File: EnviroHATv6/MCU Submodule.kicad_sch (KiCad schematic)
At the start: 10 parts, among them J1 Conn_01x10_Pin, J2 Conn_01x32_Socket, J3 Conn_01x32_Socket, U1 STM32F051R8Tx, U2 FT234XD-R, U3 CAT24C256

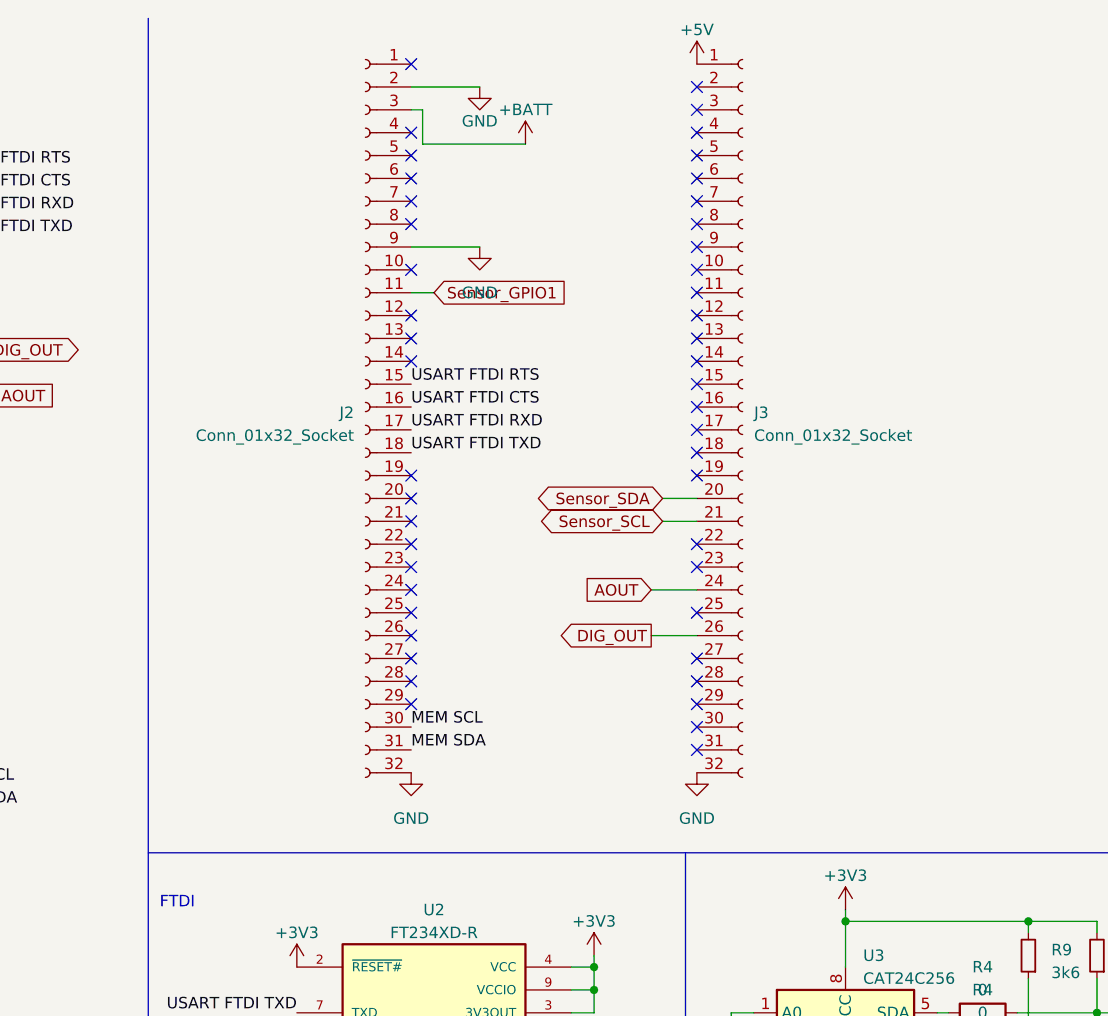
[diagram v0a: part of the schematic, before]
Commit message: Update to v 6.2
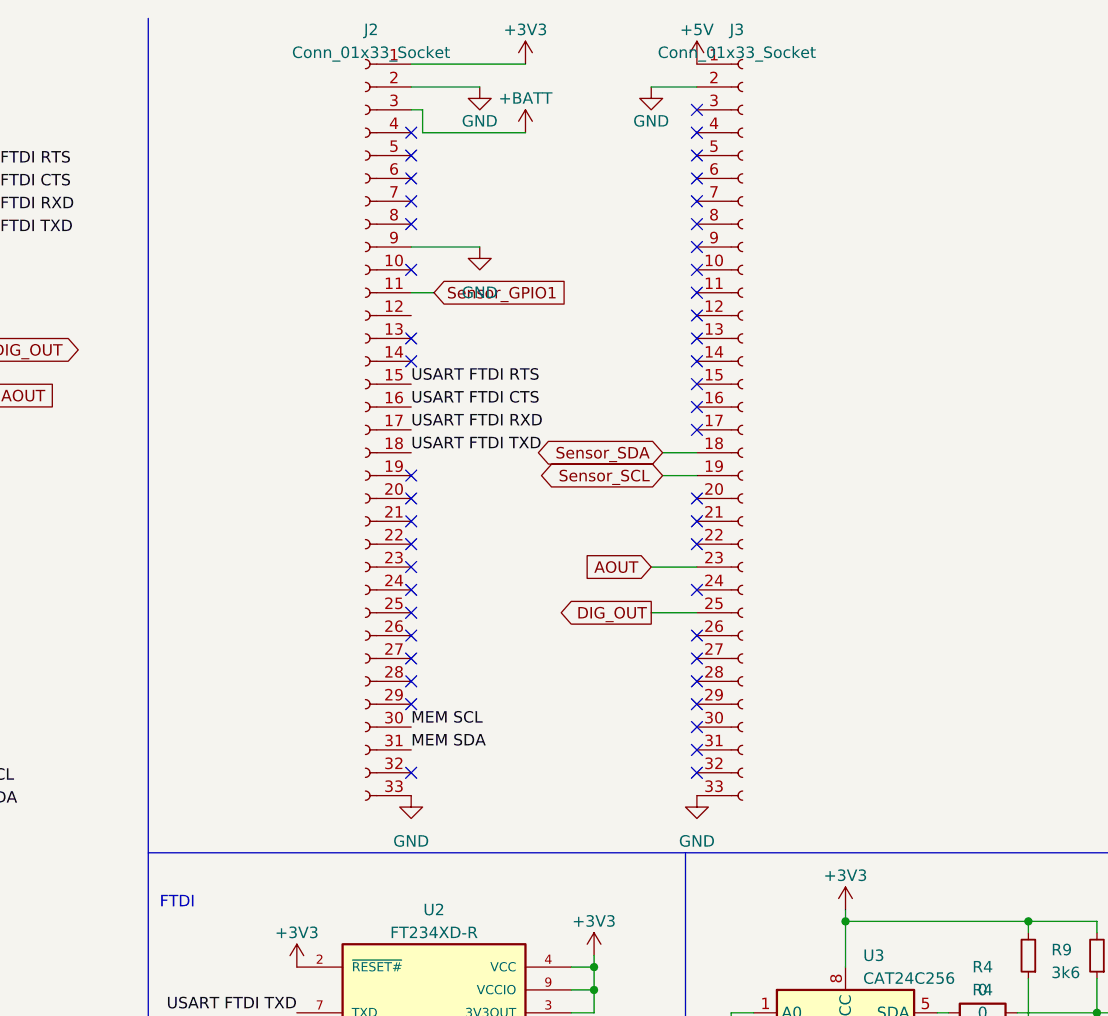
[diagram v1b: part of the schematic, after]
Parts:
- removed J2, J3: Conn_01x32_Socket, Connector_PinSocket_2.54mm:PinSocket_1x32_P2.54mm_Vertical, symbol Connector:Conn_01x32_Socket
- added J2, J3: Conn_01x33_Socket, Connector_PinSocket_2.54mm:PinSocket_1x33_P2.54mm_Vertical, symbol Connector:Conn_01x33_Socket
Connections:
- net +3V3: now also J2.1 (Pin_1)
- net +5V: now also J3.1 (Pin_1)
- net +BATT: now also J2.3 (Pin_3)
- net AOUT: now also J3.23 (Pin_23)
- net DIG_OUT: now also J3.25 (Pin_25)
- net GND: now also J2.2 (Pin_2), J2.33 (Pin_33), J2.9 (Pin_9), J3.2 (Pin_2), J3.33 (Pin_33)
- net MEM SCL: now also J2.30 (Pin_30)
- net MEM SDA: now also J2.31 (Pin_31)
- net Sensor_GPIO1: now also J2.11 (Pin_11)
- net Sensor_SCL: now also J3.19 (Pin_19)
- net Sensor_SDA: now also J3.18 (Pin_18)
- net USART FTDI CTS: now also J2.16 (Pin_16)
- net USART FTDI RTS: now also J2.15 (Pin_15)
- net USART FTDI RXD: now also J2.17 (Pin_17)
- net USART FTDI TXD: now also J2.18 (Pin_18)
- no-connect marks 93 -> 92

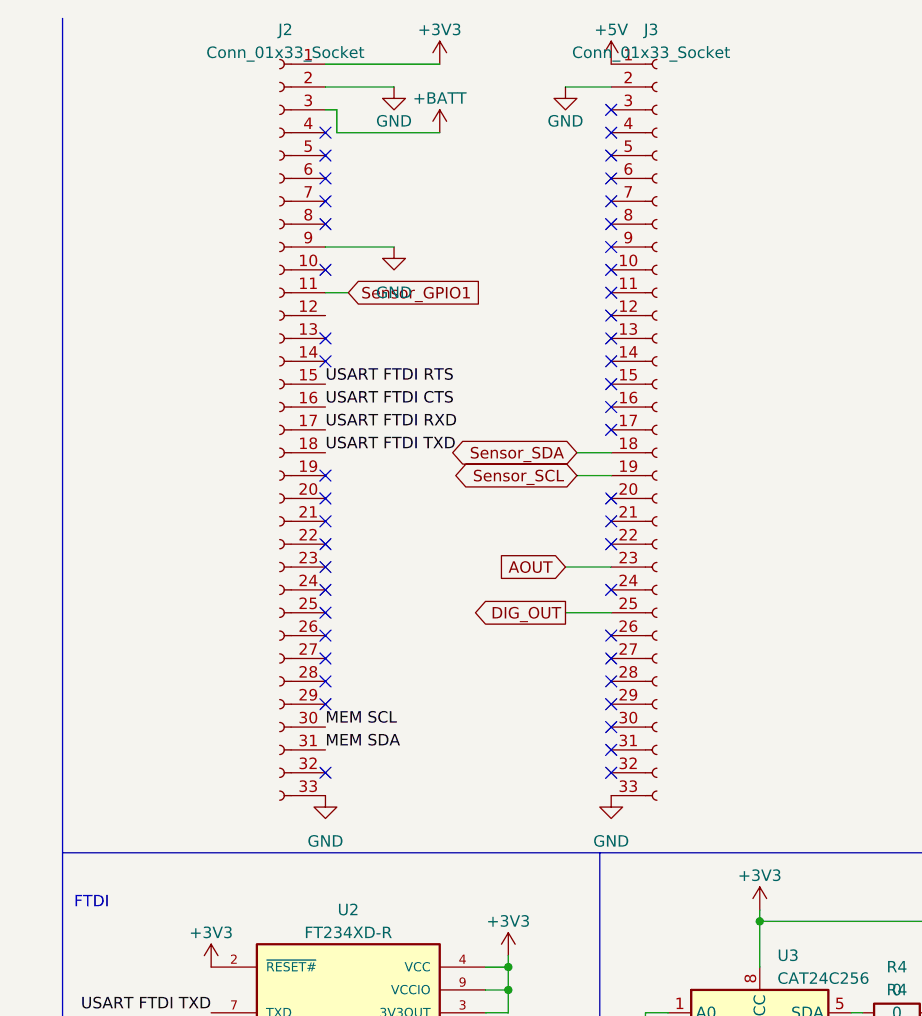
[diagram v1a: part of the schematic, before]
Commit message: PCB Cleanup V6.3
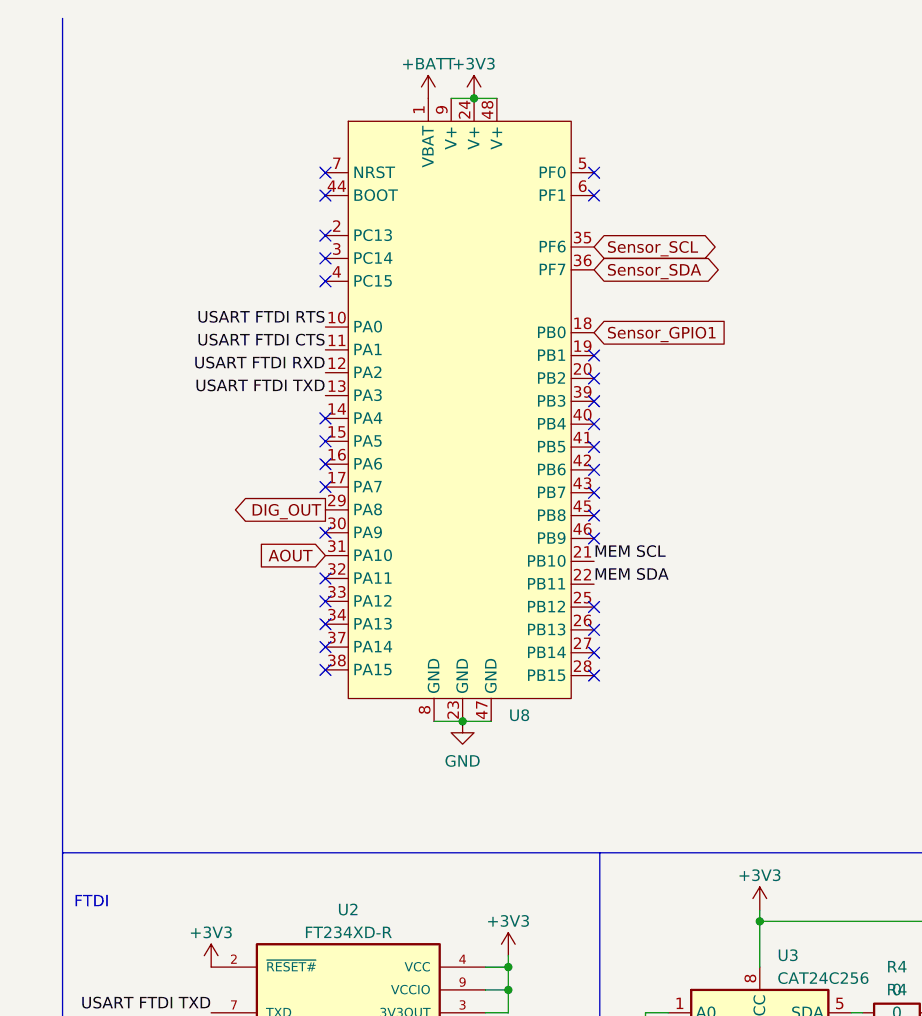
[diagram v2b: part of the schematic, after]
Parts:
- removed J2, J3: Conn_01x33_Socket, Connector_PinSocket_2.54mm:PinSocket_1x33_P2.54mm_Vertical, symbol Connector:Conn_01x33_Socket
- added U8: ~, footprints:STM32F051C6T6, symbol UCT:STM32F051C6TG6_Target
- J1: now left out of the parts list
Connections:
- net +3V3: now also U8.24 (V+), U8.48 (V+), U8.9 (V+)
- net +BATT: now also U8.1 (VBAT)
- net AOUT: now also U8.31 (PA10)
- net DIG_OUT: now also U8.29 (PA8)
- net GND: now also U8.23 (GND), U8.47 (GND), U8.8 (GND)
- net MEM SCL: now also U8.21 (PB10)
- net MEM SDA: now also U8.22 (PB11)
- net Sensor_GPIO1: now also U8.18 (PB0)
- net Sensor_SCL: now also U8.35 (PF6)
- net Sensor_SDA: now also U8.36 (PF7)
- net USART FTDI CTS: now also U8.11 (PA1)
- net USART FTDI RTS: now also U8.10 (PA0)
- net USART FTDI RXD: now also U8.12 (PA2)
- net USART FTDI TXD: now also U8.13 (PA3)
- no-connect marks 92 -> 76
